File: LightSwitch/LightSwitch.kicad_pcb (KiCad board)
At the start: 2 copper layers, 56.5 x 47.5 mm, 16 parts, among them J1 Door sensor, J2 Light switch, J3 AC input, J4 Light bulb, U1 ATMEGA328P-PU, U2 NRF24L01, U3 G3MB-202P

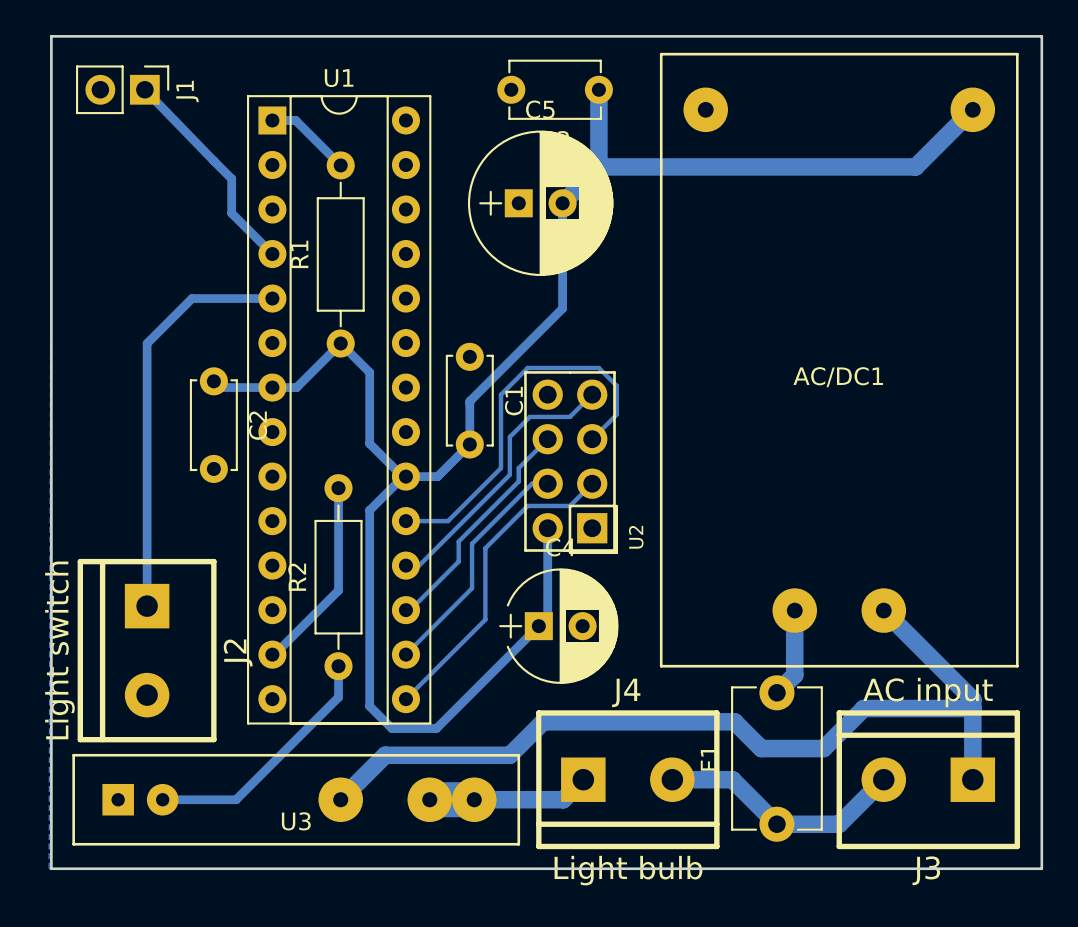
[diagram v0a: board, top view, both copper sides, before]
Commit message: LightSwitch changes
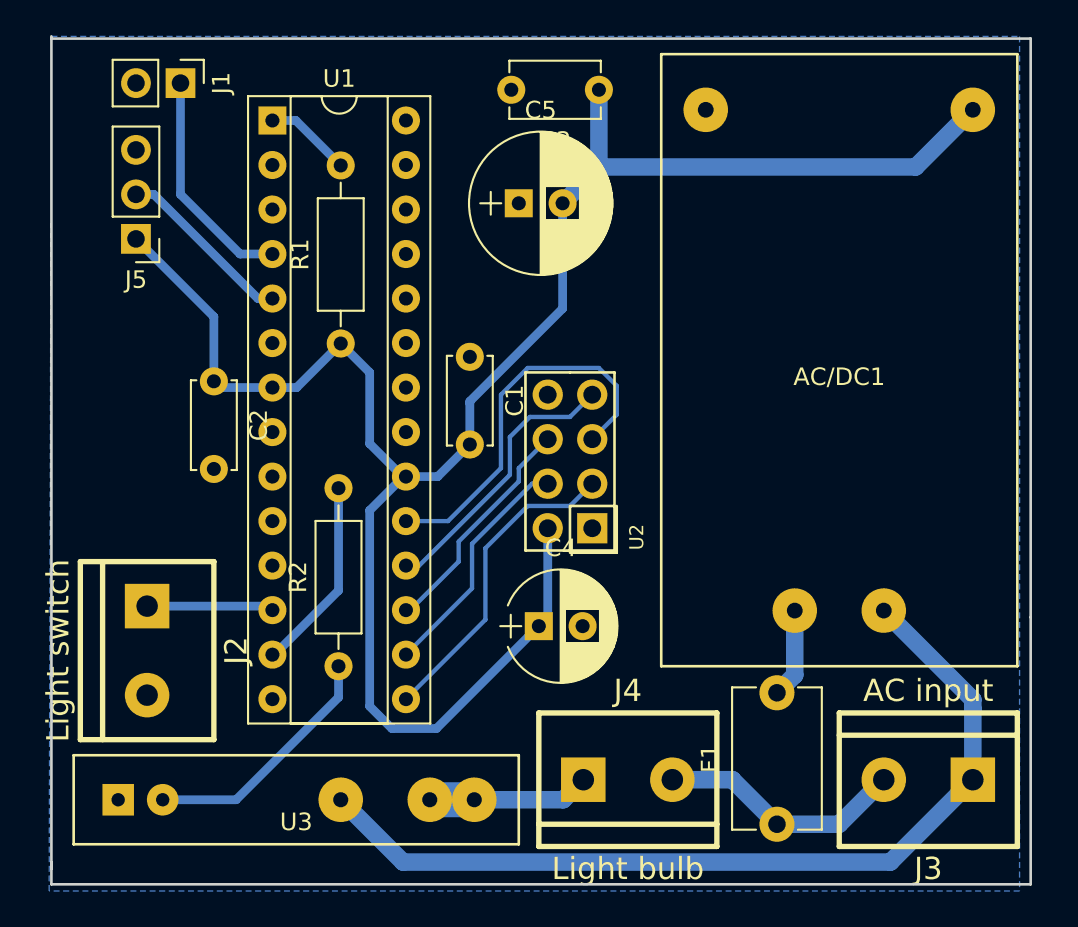
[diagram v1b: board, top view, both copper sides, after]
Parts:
- added J5: PIR sensor, Pin_Headers:Pin_Header_Straight_1x03_Pitch2.54mm, F.Cu at (140.7, 111.8)
- moved J1 2.07 mm to (143.3, 102.9)
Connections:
- U1 pad 12: (no net) -> Net-(J2-Pad1)
- U1 pad 5: Net-(J2-Pad1) -> Net-(J5-Pad2)
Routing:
- net Net-(J2-Pad1): track 23.2 -> 7.24 mm
- net Net-(J5-Pad2): track 0.00 -> 10.2 mm
- net +3V3: track 100.5 -> 110.5 mm
- net Net-(J1-Pad1): track 12.4 -> 13.0 mm
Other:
- board size 56.5 x 47.5 mm -> 55.9 x 48.4 mm
